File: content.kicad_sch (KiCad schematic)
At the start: 0 parts

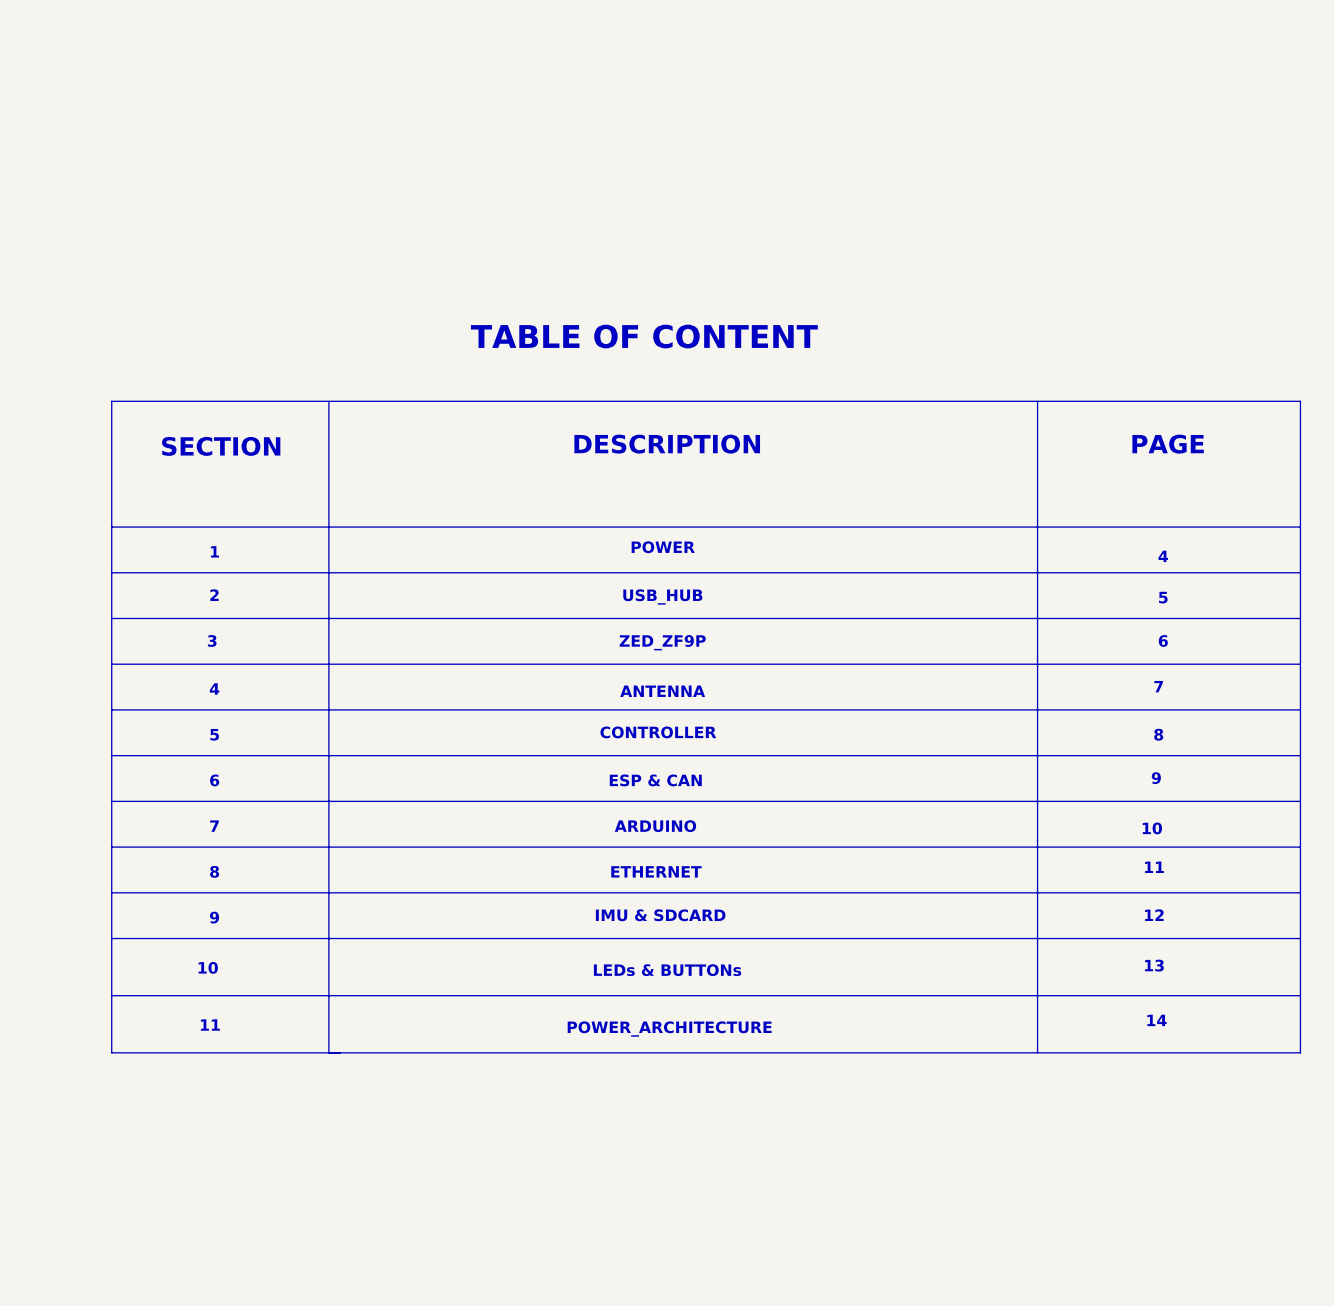
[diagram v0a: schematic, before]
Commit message: new
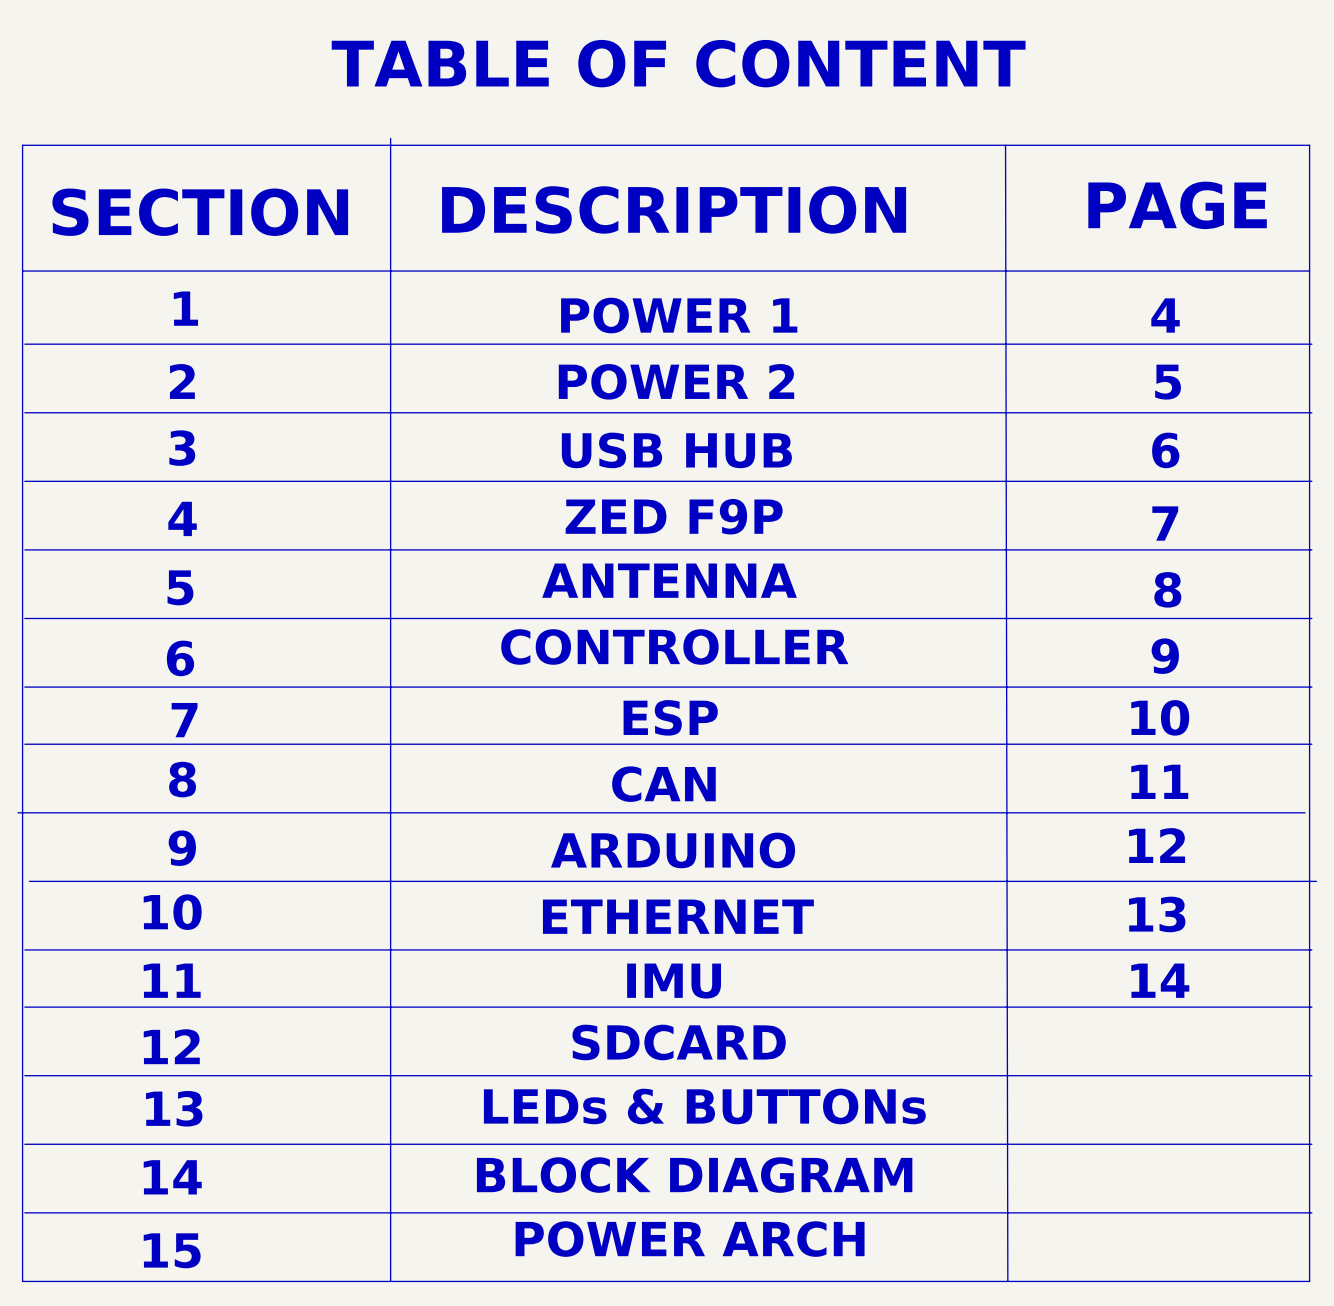
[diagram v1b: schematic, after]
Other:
- note added: "15"
- note added: "BLOCK DIAGRAM"
- note added: "CAN"
- note added: "ESP"
- note added: "IMU"
- note added: "POWER 1"
- note added: "POWER 2"
- note added: "POWER ARCH"
- note added: "SDCARD"
- note added: "USB HUB"
- note added: "ZED F9P"
- note removed: "ESP & CAN"
- note removed: "IMU & SDCARD"
- note removed: "POWER"
- note removed: "POWER_ARCHITECTURE"
- note removed: "USB_HUB"
- note removed: "ZED_ZF9P"
